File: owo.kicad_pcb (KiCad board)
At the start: 6 copper layers, 135 parts, among them J1 SJ-43516-SMT-TR, J2 SJ-43516-SMT-TR, J3 5051102291, J4 503398-1892, J5 3.7V, J6 USB4110GFA, Q1 PMOS, Q2 NMOS, SW1 KMR221GLFS, SW2 KMR221GLFS, SW3 KMR221GLFS, SW4 KMR221GLFS, SW5 KMR221GLFS, SW6 KMR221GLFS, SW7 KMR221GLFS, U1 BQ24074RGT, U10 MCP23017_ML, U11 ESP32-C6-WROOM-1, U12 KMR241GLFS, U13 KMR241GLFS, U14 OPA1622, U2 TPS7A20xxxDQN, U3 LM27762, U4 TPS62840DLCR, U5 CD74HC4067M, U6 PCM5122PW, U7 OPA1622, U8 KMR241GLFS, U9 KMR241GLFS, X1 ASE-45.1584MHz, X2 ASE-24.576MHz, Y1 32.768kHz 9pF

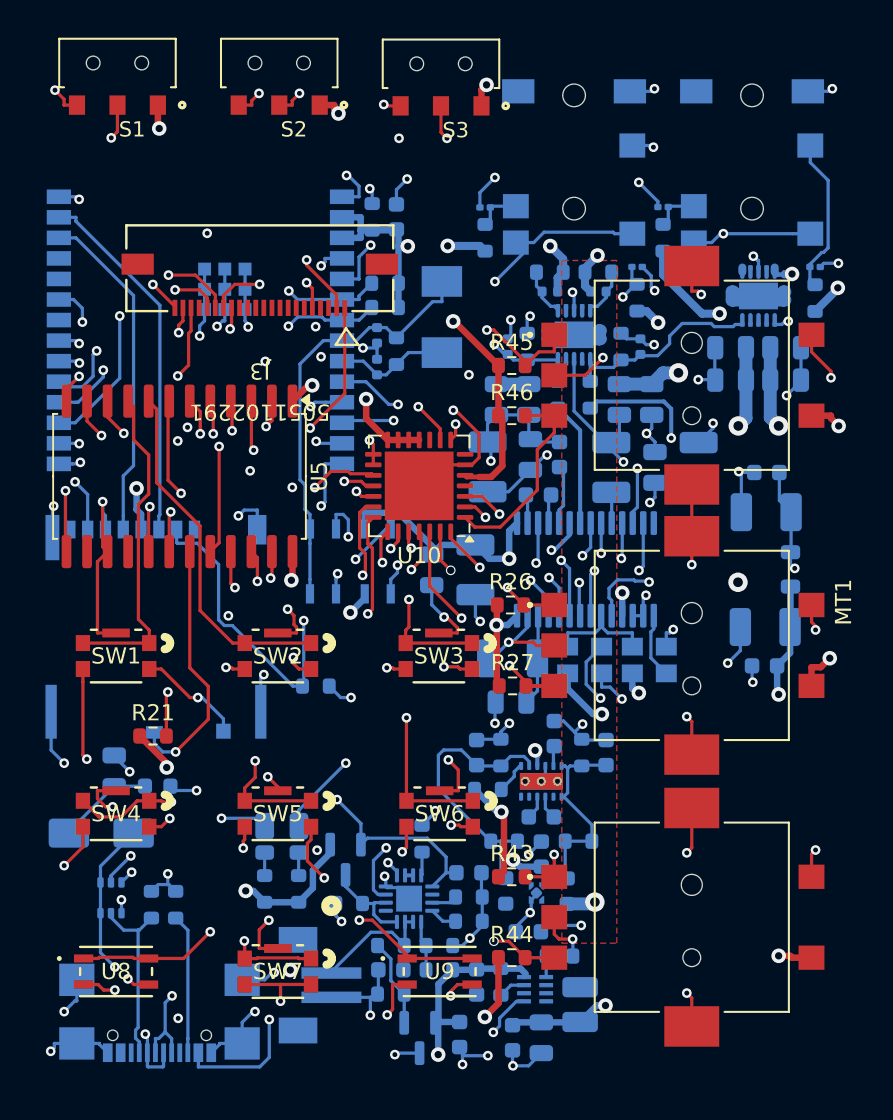
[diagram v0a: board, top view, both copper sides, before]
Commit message: more routing
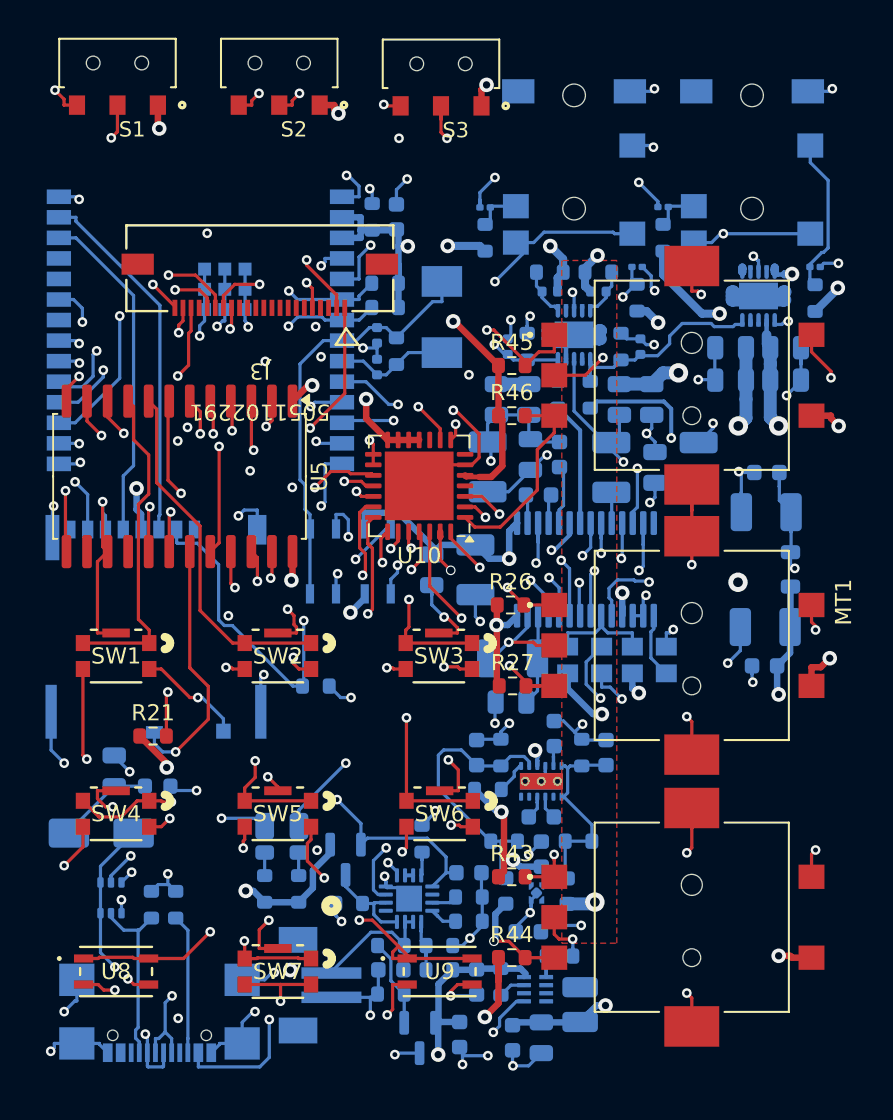
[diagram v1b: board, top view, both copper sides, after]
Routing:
- net GND: track 237.5 -> 253.5 mm
- net V5N_ANA: track 62.7 -> 72.1 mm
- net AGND: track 92.7 -> 101.4 mm
- net V3.3_SYS: track 104.5 -> 113.1 mm
- net V3.3_ANA: track 35.4 -> 39.1 mm
- net V5P_ANA: track 42.1 -> 45.7 mm
- net BTN_9: track 33.2 -> 35.1 mm
- net PCM_ATT: track 27.5 -> 28.8 mm
- net BAT_TEMP: track 3.09 -> 4.42 mm
- net LINEOUT_R: track 18.3 -> 19.1 mm
- net SWITCH_3: track 29.6 -> 30.5 mm
- net Net-(U6-SCK): track 6.73 -> 7.48 mm
- net FILTERED_L: track 12.8 -> 13.5 mm
- net ENC2_SW1: track 46.7 -> 47.4 mm
- net Net-(R22-+): track 1.30 -> 1.95 mm
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
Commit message: non ci sono parole adatte a descrivere la mia sofferenza
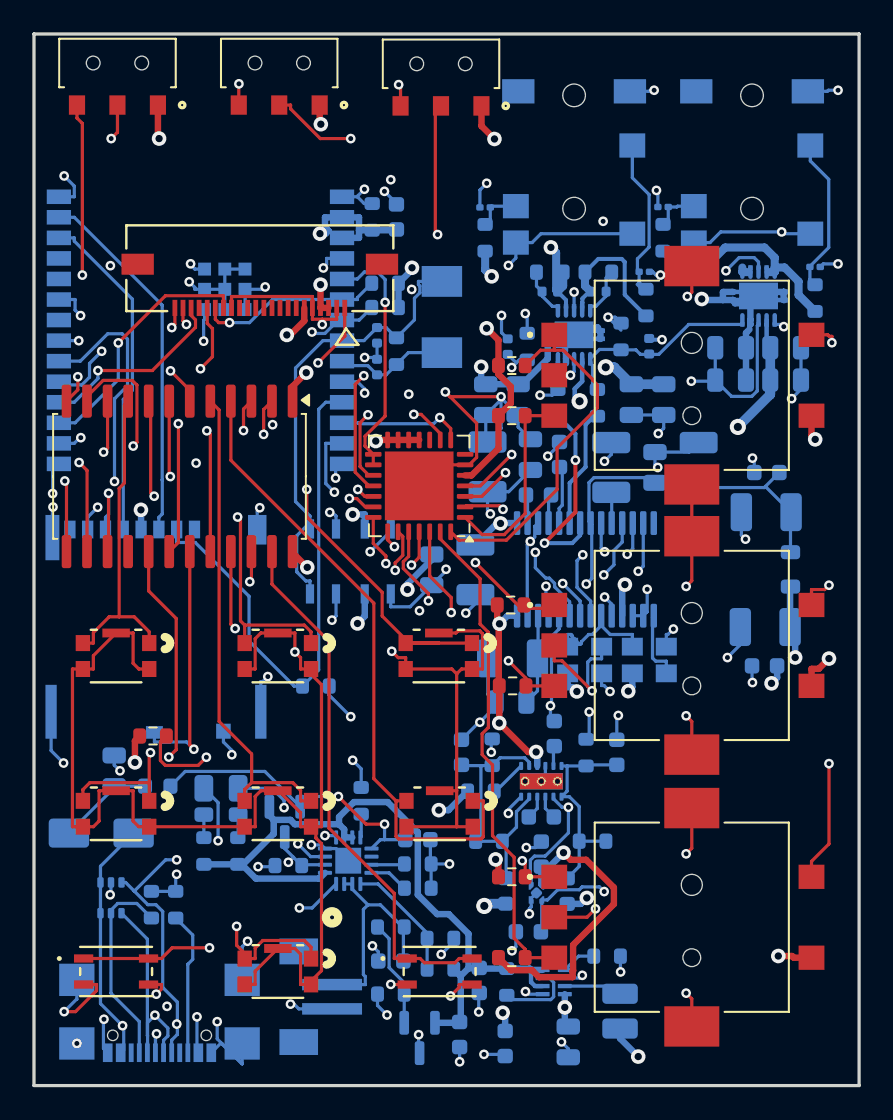
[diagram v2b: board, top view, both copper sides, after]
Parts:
- moved R1 4.43 mm to (98.6, 84.1)
- moved R4 4.43 mm to (94.1, 88.1)
- moved U1 4.43 mm to (97.8, 87.8)
- moved R19 4.43 mm to (91.0, 87.2)
- moved D1 4.43 mm to (88.9, 84.0)
- moved D2 4.43 mm to (91.0, 84.0)
- moved Q1 4.43 mm to (93.9, 85.4)
- moved R18 4.43 mm to (88.9, 87.2)
- moved C18 3.76 mm to (102.1, 86.5)
- moved R2 3.76 mm to (102.1, 89.5)
- moved R3 3.76 mm to (102.1, 88.0)
- moved R22 2.94 mm to (113.8, 93.7)
- moved L1 2.50 mm to (114.6, 97.1)
- moved C2 1.68 mm to (111.4, 99.0)
- moved U4 1.23 mm to (110.5, 95.3)
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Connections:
- net BUCK renamed Net-(L1-+)
- C10 pad 1: GND -> AGND
- C13 pad 2: GND -> AGND
- C16 pad 1: GND -> AGND
- C17 pad 1: GND -> AGND
- C18 pad 1: GND -> AGND
- C2 pad 1: GND -> AGND
- C27 pad 1: GND -> AGND
- C28 pad 1: GND -> AGND
- C3 pad 1: GND -> AGND
- C32 pad 1: GND -> AGND
- C33 pad 2: GND -> AGND
- C34 pad 2: GND -> AGND
- C35 pad 2: GND -> AGND
- C42 pad 1: GND -> AGND
- C43 pad 1: GND -> AGND
- C50 pad 2: GND -> AGND
- C6 pad 1: GND -> AGND
- D9 pad 2: GND -> AGND
- FB3 pad 2: V5N_ANA -> V5P_ANA
- J4 pad 6: GND -> AGND
- J4 pad 9: GND -> AGND
- J4 pad P1: GND -> AGND
- J4 pad P2: GND -> AGND
- J4 pad P3: GND -> AGND
- J4 pad P4: GND -> AGND
- J5 pad 2: GND -> AGND
- J6 pad A1/B12: GND -> AGND
- J6 pad B1/A12: GND -> AGND
- J6 pad S1: GND -> AGND
- J6 pad S2: GND -> AGND
- J6 pad S3: GND -> AGND
- J6 pad S4: GND -> AGND
- MT1 pad C: GND -> AGND
- MT1 pad SH1: GND -> AGND
- MT1 pad SH2: GND -> AGND
- MT2 pad B: V5N_ANA -> ENC2_B
- MT2 pad C: GND -> AGND
- MT2 pad SH1: GND -> AGND
- MT2 pad SH2: GND -> AGND
- MT3 pad C: GND -> AGND
- MT3 pad SH1: GND -> AGND
- MT3 pad SH2: GND -> AGND
- R1 pad 2: GND -> AGND
- R2 pad 2: GND -> AGND
- R22 pad 2: GND -> AGND
- R3 pad 2: GND -> AGND
- R35 pad 2: GND -> AGND
- R36 pad 2: GND -> AGND
- R37 pad 1: GND -> AGND
- R4 pad 2: GND -> AGND
- R44 pad 2: V5N_ANA -> ENC2_B
- R47 pad 2: GND -> AGND
- R48 pad 2: GND -> AGND
- S1 pad 3: GND -> AGND
- S2 pad 3: GND -> AGND
- S3 pad 3: GND -> AGND
- TH1 pad 2: GND -> AGND
- U1 pad 17: GND -> AGND
- U1 pad 8: GND -> AGND
- U10 pad 27: V5N_ANA -> ENC2_B
- U10 pad 29: GND -> AGND
- U10 pad 6: GND -> AGND
- U11 pad 1: GND -> AGND
- U11 pad 28: GND -> AGND
- U11 pad 29: GND -> AGND
- U12 pad 2: GND -> AGND
- U12 pad 3: GND -> AGND
- U13 pad 2: GND -> AGND
- U13 pad 3: GND -> AGND
- U4 pad 1: GND -> AGND
- U4 pad 6: GND -> AGND
- U5 pad 12: GND -> AGND
- U5 pad 15: GND -> AGND
- U6 pad 16: GND -> AGND
- U6 pad 17: GND -> AGND
- U6 pad 24: GND -> AGND
- U6 pad 27: GND -> AGND
- U8 pad 2: GND -> AGND
- U8 pad 3: GND -> AGND
- U9 pad 2: GND -> AGND
- U9 pad 3: GND -> AGND
- X1 pad 4: GND -> AGND
- X2 pad 4: GND -> AGND
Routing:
- net AGND: track 101.4 -> 252.4 mm, vias 21 -> 92
- net GND: track 253.5 -> 151.2 mm, vias 83 -> 4
- net DEMUX_S2: track 0.00 -> 37.2 mm, vias 0 -> 2
- net ENC2_B: track 0.00 -> 30.6 mm
- net V3.3_ANA: track 39.1 -> 62.8 mm, vias 5 -> 3
- net V5P_ANA: track 45.7 -> 66.3 mm, vias 3 -> 4
- net I2S_BCK: track 42.0 -> 62.1 mm, vias 2 -> 3
- net PCM_OUTL: track 20.1 -> 7.23 mm, vias 2 -> 0
- net AUDIO_EN: track 0.00 -> 12.8 mm, vias 0 -> 2
- net V5N_ANA: track 72.1 -> 82.3 mm, vias 4 -> 3
- net ESP_SDA: track 46.7 -> 56.3 mm
- net VSYS: track 37.8 -> 46.6 mm, vias 3 -> 0
- net Net-(U6-GPIO6/FLT): track 15.8 -> 8.74 mm
- net PMIC_PGOOD: track 17.6 -> 10.6 mm
- net I2S_WS: track 40.0 -> 47.0 mm
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- added copper zone on In1.Cu, net AGND
- removed copper zone on In1.Cu, net GND
- removed copper zone on In4.Cu, net GND
- removed copper zone on F.Cu, net V3.3_ANA
- removed copper zone on In3.Cu, net V3.3_ANA
- removed copper zone on In3.Cu, net V5N_ANA
- removed copper zone on In3.Cu, net V5P_ANA
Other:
- board outline added: 51 x 65 mm
